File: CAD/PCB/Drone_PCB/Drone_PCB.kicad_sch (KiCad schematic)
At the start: 68 parts, among them J1 MicroSD Holder, J10 UART1, J13 BATTERY, J2 MicroUSB Connector, J3 DEBUG, J4 CAM/SPI0, J5 ESP8266_WIFI, J6 M1, J7 M2, J8 M3, J9 M4, SW1 Button, SW2 Button, SW3 WiFi_RESET, SW4 UP, SW5 DOWN, U1 RP2040, U2 3V3 Regulator, U3 ICM-20948, U4 5V Regulator, U5 W25Q128JVSIQ TR, U6 Distance Sensor, U7 1V8 Regulator, Y1 12MHz

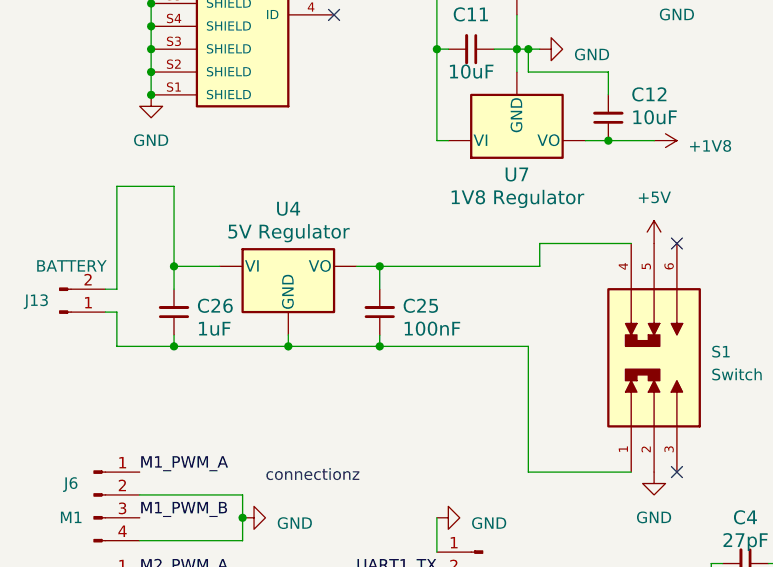
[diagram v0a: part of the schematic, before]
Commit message: finished PCB V2
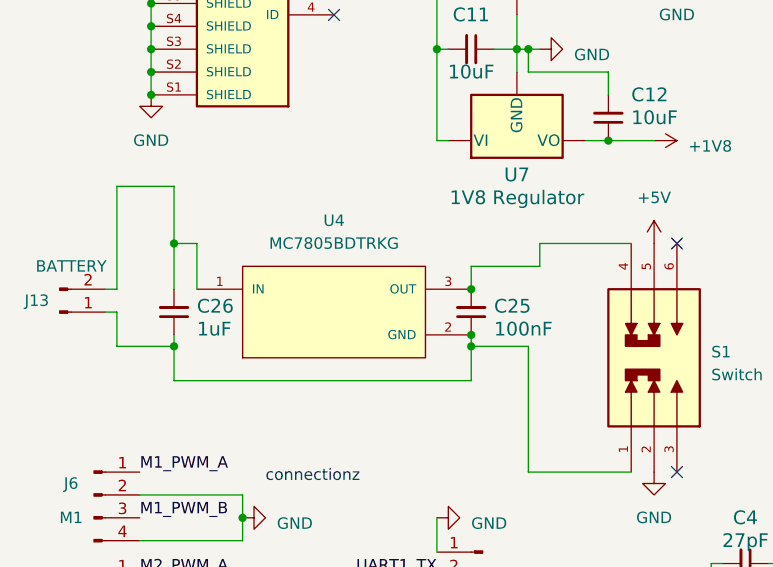
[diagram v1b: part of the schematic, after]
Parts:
- removed U4: 5V Regulator, L78L05ABUTR:SOT-89_STM, symbol Voltage Regulators:5V Regulator
- added U4: MC7805BDTRKG, DPAK229P990X238-4N, symbol MC7805BDTRKG:MC7805BDTRKG
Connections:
- net at C25.1, C26.1, J13.1 (Pin_1)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: now also U4.2 (GND)
- net at C26.2, J13.2 (Pin_2): now also U4.1 (IN)
- net at C25.2, S1.4: now also U4.3 (OUT)
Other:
- moved on the sheet: C25
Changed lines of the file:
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@@
   (junction (at 76.2 153.67) (diameter 0) (color 0 0 0 0)
   )
+  (junction (at 64.77 83.82) (diameter 0) (color 0 0 0 0)
+  )
   (junction (at 208.28 113.03) (diameter 0) (color 0 0 0 0)
   )
@@
   (junction (at 157.48 58.42) (diameter 0) (color 0 0 0 0)
   )
-  (junction (at 165.1 58.42) (diameter 0) (color 0 0 0 0)
+  (junction (at 64.77 85.09) (diameter 0) (color 0 0 0 0)
   )
-  (junction (at 54.61 85.09) (diameter 0) (color 0 0 0 0)
+  (junction (at 165.1 58.42) (diameter 0) (color 0 0 0 0)
   )
   (junction (at 275.59 140.97) (diameter 0) (color 0 0 0 0)
@@
   (junction (at 270.51 97.79) (diameter 0) (color 0 0 0 0)
   )
-  (junction (at 44.45 85.09) (diameter 0) (color 0 0 0 0)
-  )
   (junction (at 99.06 119.38) (diameter 0) (color 0 0 0 0)
   )
@@
   (junction (at 29.21 46.99) (diameter 0) (color 0 0 0 0)
   )
-  (junction (at 31.75 76.2) (diameter 0) (color 0 0 0 0)
-  )
   (junction (at 151.13 60.96) (diameter 0) (color 0 0 0 0)
   )
   (junction (at 35.56 173.99) (diameter 0) (color 0 0 0 0)
   )
-  (junction (at 54.61 76.2) (diameter 0) (color 0 0 0 0)
-  )
   (junction (at 140.97 60.96) (diameter 0) (color 0 0 0 0)
   )
   (junction (at 139.7 53.34) (diameter 0) (color 0 0 0 0)
   )
+  (junction (at 31.75 73.66) (diameter 0) (color 0 0 0 0)
+  )
   (junction (at 129.54 50.8) (diameter 0) (color 0 0 0 0)
   )
@@
   (junction (at 254 39.37) (diameter 0) (color 0 0 0 0)
   )
+  (junction (at 64.77 78.74) (diameter 0) (color 0 0 0 0)
+  )
   (junction (at 149.86 60.96) (diameter 0) (color 0 0 0 0)
   )
@@
     (stroke (width 0) (type default))
   )
+  (wire (pts (xy 34.29 73.66) (xy 31.75 73.66))
+    (stroke (width 0) (type default))
+  )
   (wire (pts (xy 53.34 163.83) (xy 54.61 163.83))
     (stroke (width 0) (type default))
@@
     (stroke (width 0) (type default))
   )
-  (wire (pts (xy 54.61 76.2) (xy 52.07 76.2))
-    (stroke (width 0) (type default))
-  )
   (wire (pts (xy 149.86 60.96) (xy 151.13 60.96))
     (stroke (width 0) (type default))
@@
     (stroke (width 0) (type default))
   )
+  (wire (pts (xy 64.77 76.2) (xy 72.39 76.2))
+    (stroke (width 0) (type default))
+  )
   (wire (pts (xy 208.28 102.87) (xy 208.28 113.03))
     (stroke (width 0) (type default))
@@
     (stroke (width 0) (type default))
   )
+  (wire (pts (xy 64.77 88.9) (xy 64.77 85.09))
+    (stroke (width 0) (type default))
+  )
   (wire (pts (xy 106.68 86.36) (xy 118.11 86.36))
     (stroke (width 0) (type default))
@@
     (stroke (width 0) (type default))
   )
-  (wire (pts (xy 31.75 67.31) (xy 31.75 76.2))
+  (wire (pts (xy 31.75 67.31) (xy 31.75 73.66))
     (stroke (width 0) (type default))
   )
@@
     (stroke (width 0) (type default))
   )
-  (wire (pts (xy 36.83 76.2) (xy 31.75 76.2))
-    (stroke (width 0) (type default))
-  )
   (wire (pts (xy 135.89 193.04) (xy 147.32 193.04))
     (stroke (width 0) (type default))
@@
     (stroke (width 0) (type default))
   )
-  (wire (pts (xy 93.98 182.88) (xy 100.33 182.88))
+  (wire (pts (xy 34.29 78.74) (xy 34.29 73.66))
     (stroke (width 0) (type default))
   )
-  (wire (pts (xy 114.49 130.81) (xy 115.57 130.81))
+  (wire (pts (xy 93.98 182.88) (xy 100.33 182.88))
     (stroke (width 0) (type default))
   )
-  (wire (pts (xy 54.61 85.09) (xy 71.12 85.09))
+  (wire (pts (xy 114.49 130.81) (xy 115.57 130.81))
     (stroke (width 0) (type default))
   )
@@
     (stroke (width 0) (type default))
   )
-  (wire (pts (xy 54.61 83.82) (xy 54.61 85.09))
+  (wire (pts (xy 64.77 83.82) (xy 64.77 85.09))
     (stroke (width 0) (type default))
   )
@@
     (stroke (width 0) (type default))
   )
-  (wire (pts (xy 44.45 85.09) (xy 54.61 85.09))
-    (stroke (width 0) (type default))
-  )
   (wire (pts (xy 76.2 158.75) (xy 59.69 158.75))
     (stroke (width 0) (type default))
@@
     (stroke (width 0) (type default))
   )
+  (wire (pts (xy 31.75 88.9) (xy 31.75 85.09))
+    (stroke (width 0) (type default))
+  )
   (wire (pts (xy 204.47 31.75) (xy 208.28 31.75))
     (stroke (width 0) (type default))
@@
     (stroke (width 0) (type default))
   )
-  (wire (pts (xy 31.75 76.2) (xy 31.75 78.74))
-    (stroke (width 0) (type default))
-  )
   (wire (pts (xy 53.34 153.67) (xy 53.34 156.21))
     (stroke (width 0) (type default))
@@
     (stroke (width 0) (type default))
   )
+  (wire (pts (xy 31.75 73.66) (xy 31.75 78.74))
+    (stroke (width 0) (type default))
+  )
   (wire (pts (xy 153.67 60.96) (xy 156.21 60.96))
     (stroke (width 0) (type default))
@@
     (stroke (width 0) (type default))
   )
+  (wire (pts (xy 64.77 85.09) (xy 71.12 85.09))
+    (stroke (width 0) (type default))
+  )
   (wire (pts (xy 25.4 166.37) (xy 45.72 166.37))
     (stroke (width 0) (type default))
@@
     (stroke (width 0) (type default))
   )
-  (wire (pts (xy 44.45 85.09) (xy 44.45 83.82))
-    (stroke (width 0) (type default))
-  )
   (wire (pts (xy 255.27 97.79) (xy 270.51 97.79))
     (stroke (width 0) (type default))
@@
     (stroke (width 0) (type default))
   )
-  (wire (pts (xy 54.61 76.2) (xy 54.61 78.74))
+  (wire (pts (xy 64.77 76.2) (xy 64.77 78.74))
     (stroke (width 0) (type default))
   )
@@
     (stroke (width 0) (type default))
   )
-  (wire (pts (xy 31.75 85.09) (xy 44.45 85.09))
+  (wire (pts (xy 31.75 88.9) (xy 64.77 88.9))
     (stroke (width 0) (type default))
   )
@@
     (stroke (width 0) (type default))
   )
-  (wire (pts (xy 54.61 76.2) (xy 72.39 76.2))
-    (stroke (width 0) (type default))
-  )
   (wire (pts (xy 27.94 106.68) (xy 39.37 106.68))
     (stroke (width 0) (type default))
@@
     )
   )
+  (symbol (lib_id "MC7805BDTRKG:MC7805BDTRKG") (at 49.53 81.28 0) (unit 1)
+    (in_bom yes) (on_board yes) (dnp no) (fields_autoplaced)
+    (property "Reference" "U4" (at 49.53 71.12 0)
+      (effects (font (size 1.27 1.27)))
+    )
+    (property "Value" "MC7805BDTRKG" (at 49.53 73.66 0)
+      (effects (font (size 1.27 1.27)))
+    )
+    (property "Footprint" "DPAK229P990X238-4N" (at 49.53 81.28 0)
+      (effects (font (size 1.27 1.27)) (justify bottom) hide)
+    )
+    (property "Datasheet" "" (at 49.53 81.28 0)
+      (effects (font (size 1.27 1.27)) hide)
+    )
+    (property "PARTREV" "27" (at 49.53 81.28 0)
+      (effects (font (size 1.27 1.27)) (justify bottom) hide)
+    )
+    (property "STANDARD" "IPC-7351B" (at 49.53 81.28 0)
+      (effects (font (size 1.27 1.27)) (justify bottom) hide)
+    )
+    (property "MANUFACTURER" "ON Semiconductor" (at 49.53 81.28 0)
+      (effects (font (size 1.27 1.27)) (justify bottom) hide)
+    )
+    (pin "1")
+    (pin "2")
+    (pin "3")
+    (instances
+      (project "Drone_PCB"
+        (path "/78662915-a4bc-47c2-ae27-aef37b2538d7"
+          (reference "U4") (unit 1)
+        )
+      )
+    )
+  )
   (symbol (lib_id "Capacitors:10uF") (at 54.61 36.83 270) (unit 1)
     (in_bom yes) (on_board yes) (dnp no) (fields_autoplaced)
@@
     )
   )
-  (symbol (lib_id "Voltage Regulators:5V Regulator") (at 44.45 77.47 0) (unit 1)
-    (in_bom yes) (on_board yes) (dnp no) (fields_autoplaced)
-    (property "Reference" "U4" (at 44.45 69.85 0)
-      (effects (font (size 1.524 1.524)))
-    )
-    (property "Value" "5V Regulator" (at 44.45 72.39 0)
-      (effects (font (size 1.524 1.524)))
-    )
-    (property "Footprint" "L78L05ABUTR:SOT-89_STM" (at 44.45 77.47 0)
-      (effects (font (size 1.27 1.27) italic) hide)
-    )
-    (property "Datasheet" "~" (at 44.45 77.47 0)
-      (effects (font (size 1.27 1.27) italic) hide)
-    )
-    (pin "1")
-    (pin "2")
-    (pin "3")
-    (instances
-      (project "Drone_PCB"
-        (path "/78662915-a4bc-47c2-ae27-aef37b2538d7"
-          (reference "U4") (unit 1)
-        )
-      )
-    )
-  )
   (symbol (lib_id "Capacitors:10uF") (at 87.63 39.37 270) (unit 1)
     (in_bom yes) (on_board yes) (dnp no) (fields_autoplaced)
@@
     )
   )
-  (symbol (lib_id "Capacitors:100nF") (at 54.61 81.28 270) (unit 1)
+  (symbol (lib_id "Capacitors:100nF") (at 64.77 81.28 270) (unit 1)
     (in_bom yes) (on_board yes) (dnp no) (fields_autoplaced)
-    (property "Reference" "C25" (at 57.15 80.6386 90)
+    (property "Reference" "C25" (at 67.31 80.6386 90)
       (effects (font (size 1.524 1.524)) (justify left))
     )
-    (property "Value" "100nF" (at 57.15 83.1786 90)
+    (property "Value" "100nF" (at 67.31 83.1786 90)
       (effects (font (size 1.524 1.524)) (justify left))
     )
-    (property "Footprint" "0402YC104KAT2A:CAPC1005X56N" (at 54.61 81.28 0)
+    (property "Footprint" "0402YC104KAT2A:CAPC1005X56N" (at 64.77 81.28 0)
       (effects (font (size 1.524 1.524)) hide)
     )
-    (property "Datasheet" "" (at 54.61 81.28 0)
+    (property "Datasheet" "" (at 64.77 81.28 0)
       (effects (font (size 1.524 1.524)))
     )
